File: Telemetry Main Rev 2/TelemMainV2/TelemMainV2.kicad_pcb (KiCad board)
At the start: 2 copper layers, 161 x 113.3 mm, 59 parts, among them J1 8 pin ATM connector, J2 40 pin ZIF FPC Connector, J3 12 pin ATM connector, J4 SD to SPI (Molex nanofit), U1 LM7805_TO220, U2 LM7809_TO220, U3 NUCLEO-F446RE, U4 ISO1050DUB, U5 XBP9B-DPST-001, U6 MCP6004, U7 BT817Q, U8 ISO1050DUB

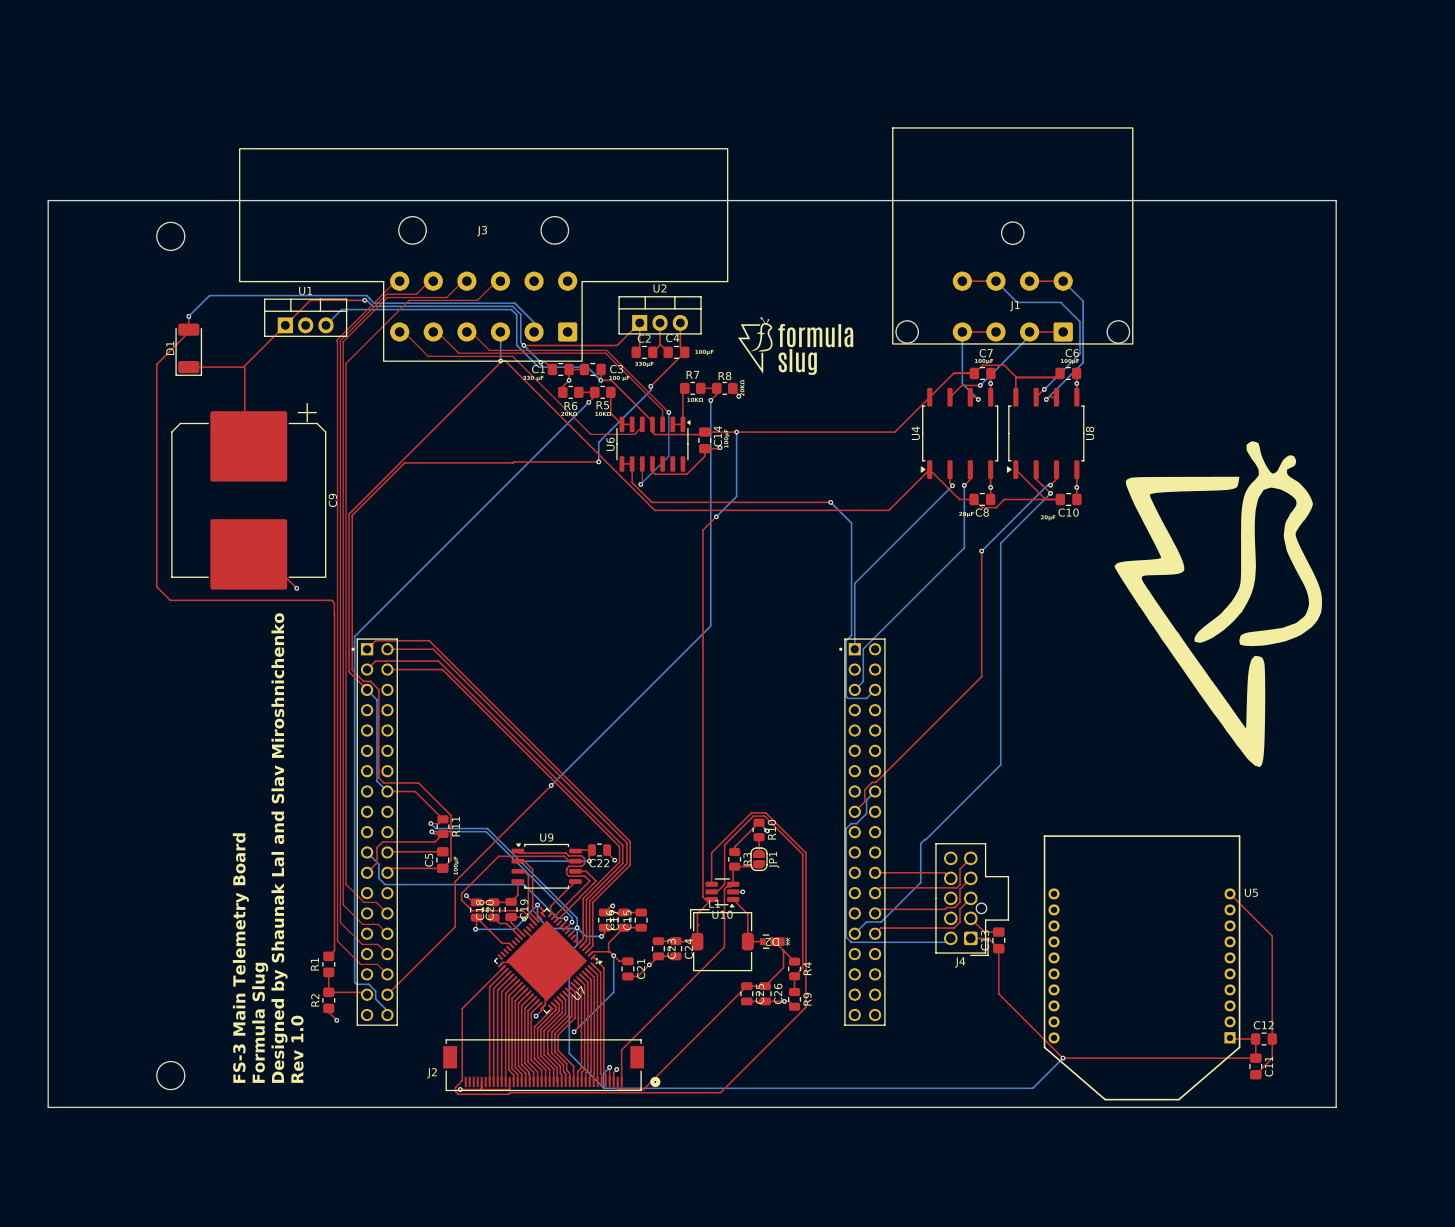
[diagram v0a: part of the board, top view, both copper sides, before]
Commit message: i had to delete half of this board and start it over again i am going to go missing soon
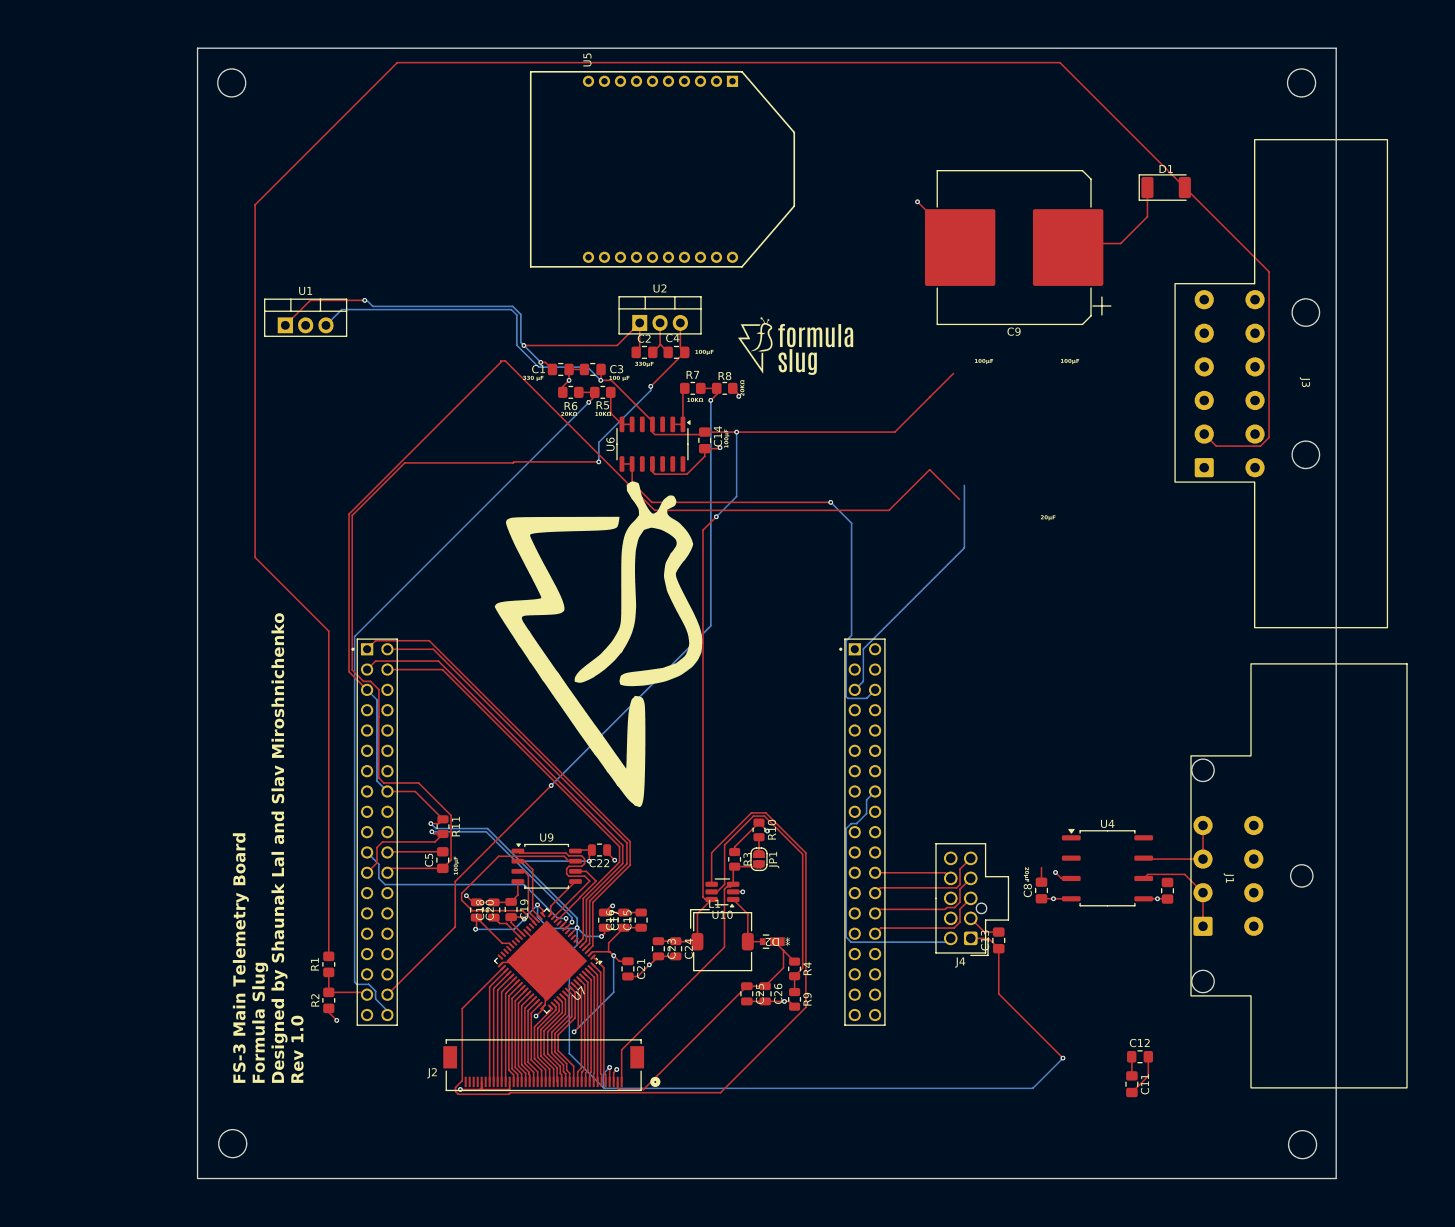
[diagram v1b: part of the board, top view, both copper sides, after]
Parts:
- removed C10, C6: 100nf, Capacitor_SMD:C_0805_2012Metric_Pad1.18x1.45mm_HandSolder
- removed the REF** at (71.2, 152.4)
- removed the REF** at (71.2, 47.5)
- removed U8: ISO1050DUB, Package_SO:SOP-8_6.62x9.15mm_P2.54mm
- added REF**: MountingHole_3.5mm, MountingHole:MountingHole_3.5mm, F.Cu at (212.6, 28.3)
- added REF**: MountingHole_3.5mm, MountingHole:MountingHole_3.5mm, F.Cu at (78.9, 28.3)
- added REF**: MountingHole_3.5mm, MountingHole:MountingHole_3.5mm, F.Cu at (79.0, 160.9)
- added REF**: MountingHole_3.5mm, MountingHole:MountingHole_3.5mm, F.Cu at (212.7, 161.0)
- moved J3 126.9 mm to (216.8, 45.4), turned to -90 degrees
- moved D1 123.8 mm to (195.7, 41.4), turned to 0 degrees
- moved U5 116.4 mm to (132.7, 39.1), turned to -90 degrees
- moved C9 100.8 mm to (176.7, 48.9), turned to 180 degrees
- moved G1 77.6 mm to (124.3, 97.9)
- moved C7 68.7 mm to (195.8, 129.3), turned to 90 degrees
- moved J1 63.6 mm to (198.8, 112.4), turned to -90 degrees
- moved U4 57.4 mm to (188.3, 126.5), turned to 0 degrees
- moved C8 49.4 mm to (180.1, 129.3), turned to 90 degrees
- moved C11 15.7 mm to (191.4, 153.5)
- moved C12 15.7 mm to (192.4, 150.1)
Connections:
- J1 pad 1: CAN1_H -> CAN1_L
- J1 pad 2: CAN1_H -> CAN1_L
- J1 pad 3: CAN1_L -> CAN1_H
- J1 pad 4: CAN1_L -> CAN1_H
- J1 pad 5: CAN2_H -> unconnected-(J1-Pin_5-Pad5)
- J1 pad 6: CAN2_H -> unconnected-(J1-Pin_6-Pad6)
- J1 pad 7: CAN2_L -> unconnected-(J1-Pin_7-Pad7)
- J1 pad 8: CAN2_L -> unconnected-(J1-Pin_8-Pad8)
- U3 pad CN10_17: CAN2_TX -> unconnected-(U3B-PB6-PadCN10_17)
- U3 pad CN10_29: CAN2_RX -> unconnected-(U3B-PB5-PadCN10_29)
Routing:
- net +12VIN: track 149.3 -> 272.6 mm, vias 1 -> 0
- net Acc Intake Pressure: track 96.2 -> 0.00 mm
- net Acc Intake Flow Rate: track 95.6 -> 0.00 mm
- net Acc Exhaust Temp: track 95.2 -> 0.00 mm
- net Acc Intake Temp: track 94.3 -> 0.00 mm
- net CAN2_RX: track 70.1 -> 0.00 mm, vias 1 -> 0
- net CAN2_TX: track 53.7 -> 0.00 mm, vias 2 -> 0
- net +3V3: track 376.3 -> 325.3 mm, vias 10 -> 9
- net Steering Sensor: track 42.7 -> 0.00 mm, vias 2 -> 0
- net Brake Sensor B: track 36.5 -> 0.00 mm
- net Brake Sensor F: track 34.7 -> 0.00 mm
- net GND: track 149.4 -> 118.9 mm, vias 19 -> 17
- net CAN2_H: track 28.5 -> 0.00 mm, vias 1 -> 0
- net CAN1_RX: track 27.6 -> 0.00 mm, vias 1 -> 0
- net +5V: track 189.9 -> 164.4 mm
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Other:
- board size 161 x 113.3 mm -> 142.3 x 141.3 mm

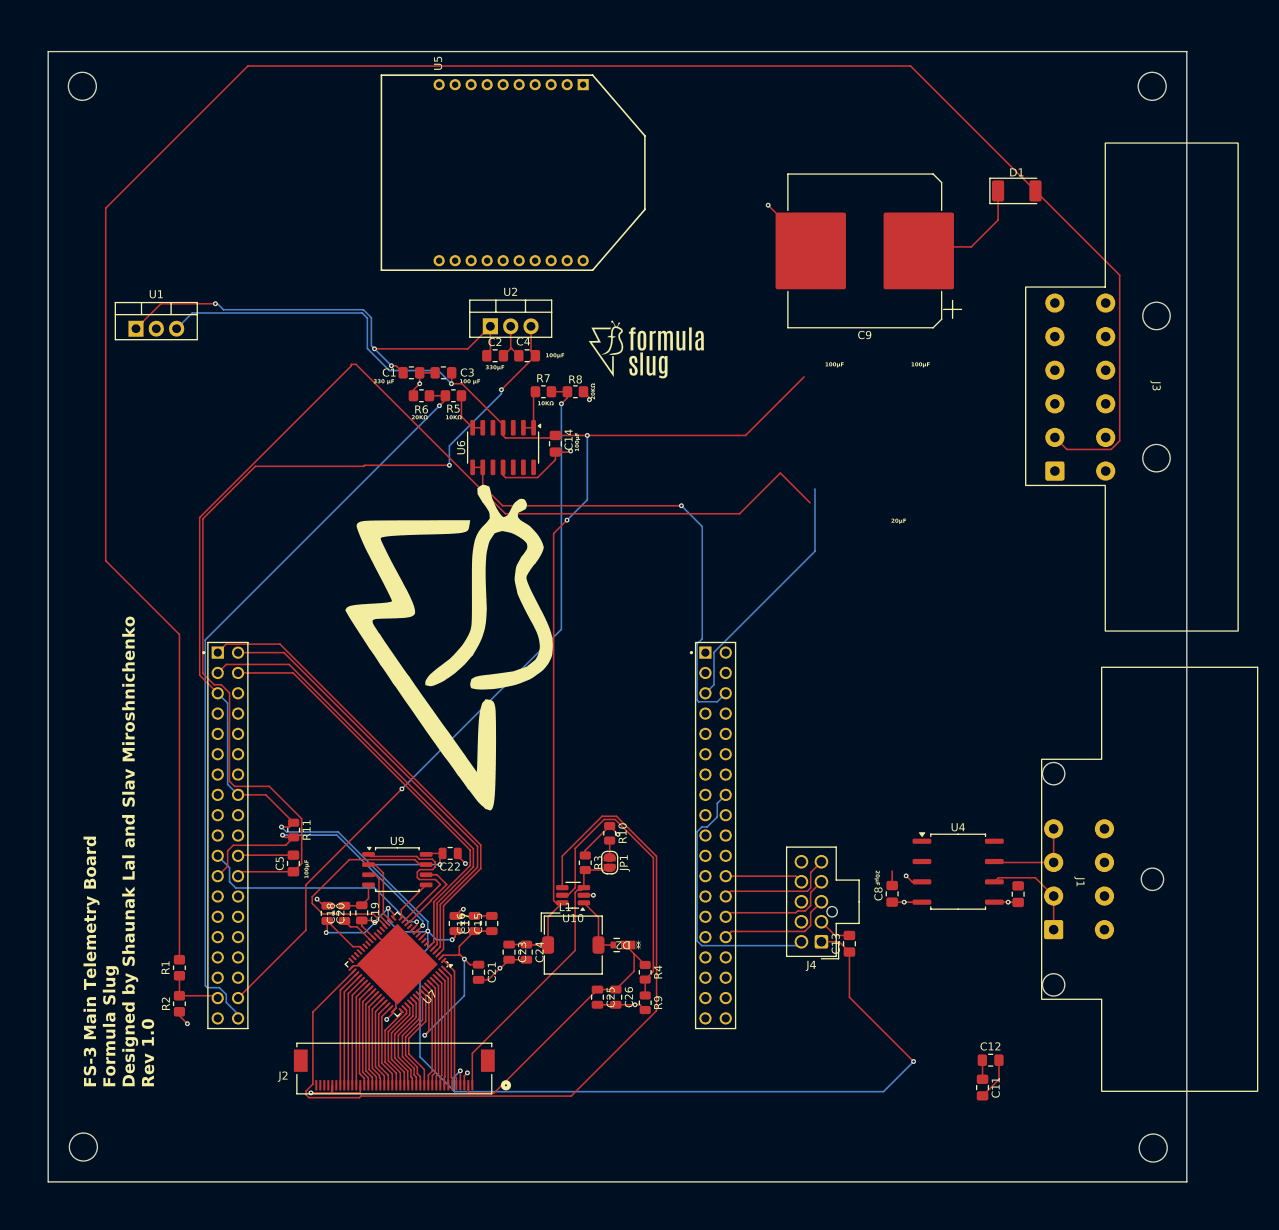
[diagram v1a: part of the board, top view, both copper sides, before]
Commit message: pushing changes from 2/18
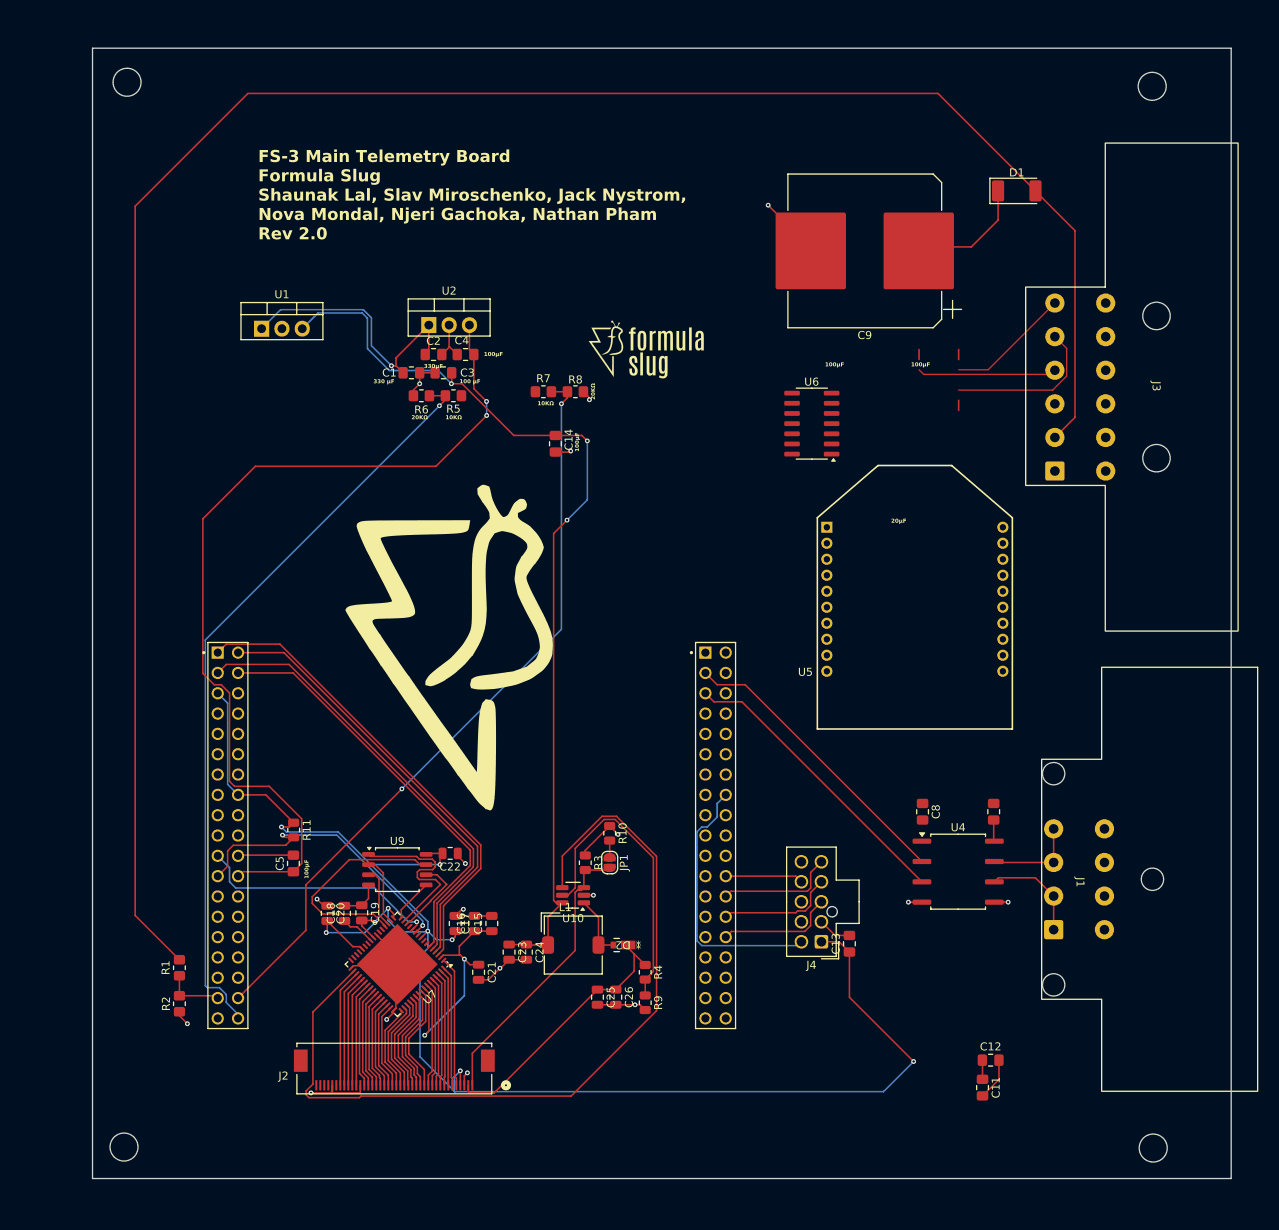
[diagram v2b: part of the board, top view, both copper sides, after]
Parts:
- moved U5 73.1 mm to (182.9, 92.2), turned to 0 degrees
- moved U6 38.7 mm to (170.1, 70.5), turned to 180 degrees
- moved U1 15.7 mm to (101.3, 58.6)
- moved C8 10.9 mm to (183.9, 119.0), turned to -90 degrees
- moved C7 10.7 mm to (192.8, 119.0), turned to -90 degrees
- moved C2 7.70 mm to (122.8, 61.8)
- moved C4 7.70 mm to (126.8, 61.8)
- moved U2 7.70 mm to (122.2, 58.2)
- moved REF** 5.61 mm to (84.5, 27.8)
- moved REF** 5.08 mm to (84.1, 160.9)
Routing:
- net +3V3: track 325.3 -> 204.8 mm
- net Steering Sensor 3V3: track 59.2 -> 1.27 mm, vias 1 -> 0
- net +5V: track 164.4 -> 120.4 mm
- net CAN1_RX: track 0.00 -> 36.8 mm
- net +12V: track 74.1 -> 48.9 mm, vias 3 -> 1
- net Brake Sensor F: track 0.00 -> 19.8 mm
- net +12VIN: track 272.6 -> 253.8 mm
- net Steering Sensor: track 0.00 -> 17.4 mm
- net Brake Sensor B: track 0.00 -> 15.5 mm
- net GND: track 118.9 -> 106.2 mm
- net Net-(U6B--): track 5.85 -> 1.27 mm
- net Net-(U6A--): track 5.54 -> 1.27 mm
- net CAN1_TX: track 33.5 -> 36.8 mm, vias 1 -> 0
- net +9V: track 115.5 -> 112.9 mm
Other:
- board text added: "FS-3 Main Telemetry Board Formula Slug Shaunak Lal, Slav Miroschenko, Jack Nystrom, Nova Mondal, Njeri Gachoka, Nathan Pham Rev 2.0"
- board text removed: "FS-3 Main Telemetry Board Formula Slug Designed by Shaunak Lal and Slav Miroshnichenko Rev 1.0"
